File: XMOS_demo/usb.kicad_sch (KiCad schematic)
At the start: 9 parts, among them J2 USB_C_Receptacle_USB2.0_16P, U4 TPD3S014

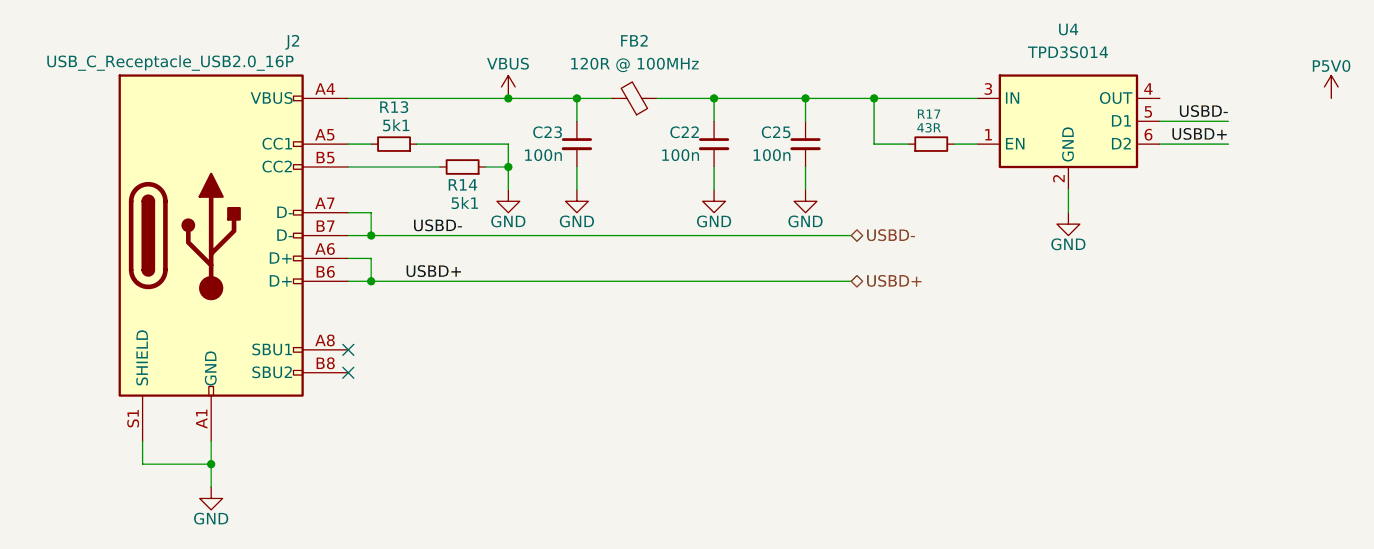
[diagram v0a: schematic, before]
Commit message: sch work
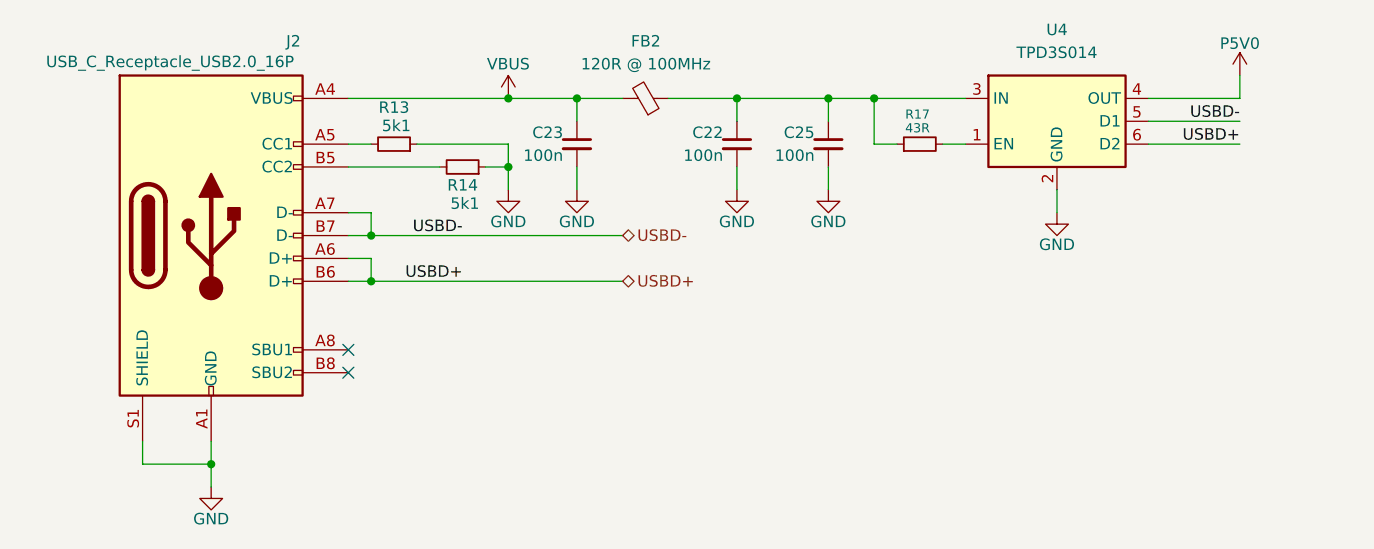
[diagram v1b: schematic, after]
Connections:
- net P5V0: now also U4.4 (OUT)
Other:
- company: (none) -> AGH University
- title: (none) -> USB Sound Card USB Port
- moved on the sheet: C22, C25, FB2, R17, U4

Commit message: Lots of sch work
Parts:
- C22, C23, C25: Max Voltage 10V -> 16V
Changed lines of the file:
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@@
 			)
 		)
-		(property "Max Voltage" "10V"
+		(property "Max Voltage" "16V"
 			(at 180.34 81.28 0)
 			(effects
@@
 			)
 		)
-		(property "Max Voltage" "10V"
+		(property "Max Voltage" "16V"
 			(at 152.4 81.28 0)
 			(effects
@@
 			)
 		)
-		(property "Max Voltage" "10V"
+		(property "Max Voltage" "16V"
 			(at 170.18 81.28 0)
 			(effects
